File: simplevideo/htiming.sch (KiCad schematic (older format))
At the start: 4 parts, among them U14 CD74HC40103, U15 CD74HC40103, U16 CD74HC40103, U17 74LS74

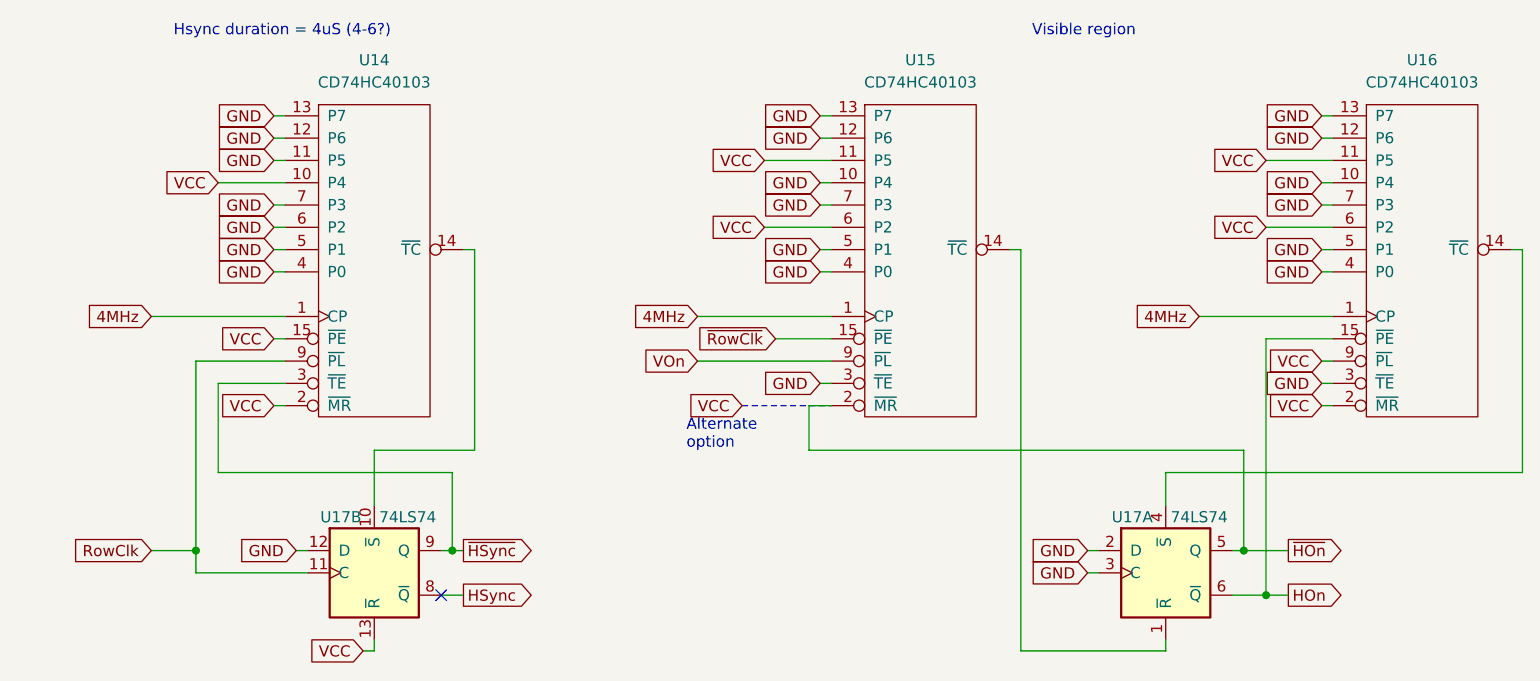
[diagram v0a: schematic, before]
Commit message: Fixed various issues discovered during building and testing
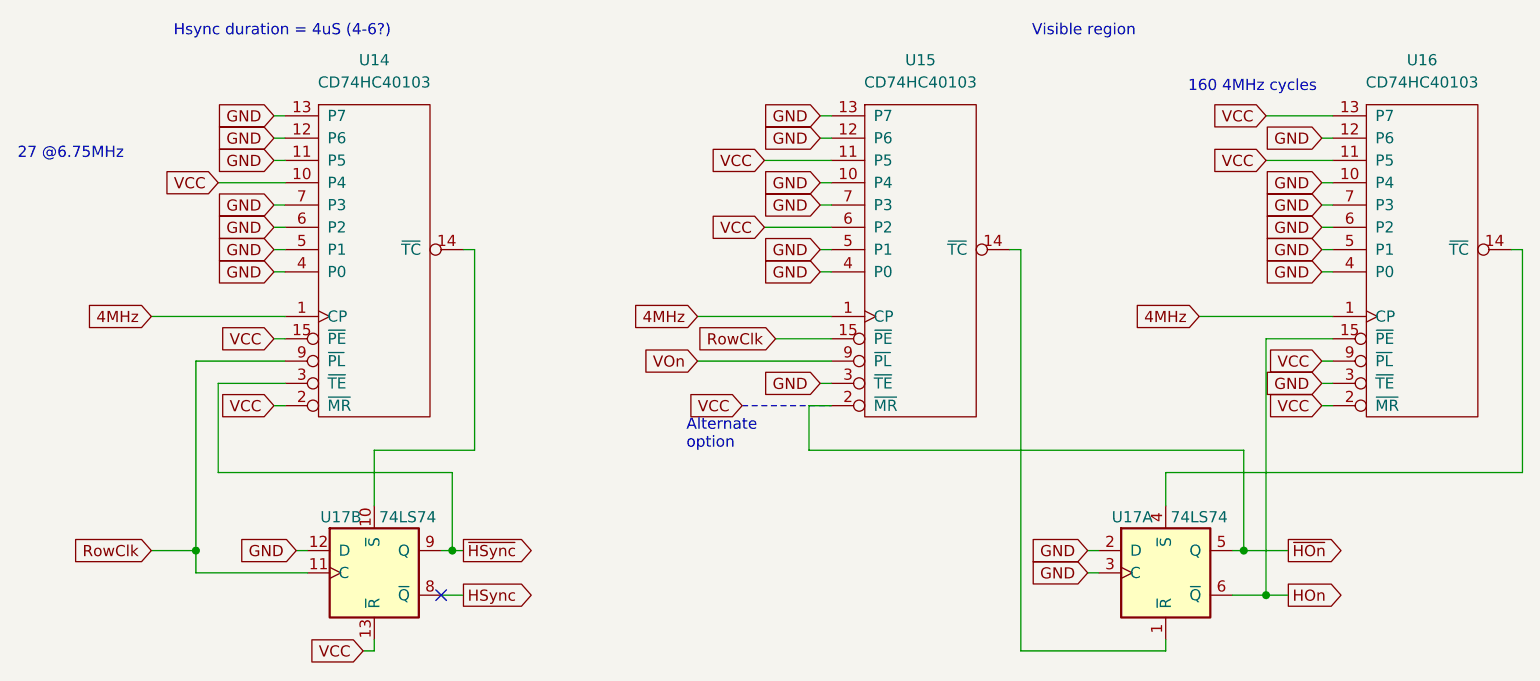
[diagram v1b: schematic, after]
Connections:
- net ~RowClk is gone; now on net RowClk: U15.15 (~PE)
- net GND: now also U16.6 (P2); no longer U16.13 (P7)
- net VCC: now also U16.13 (P7); no longer U16.6 (P2)
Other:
- note added: "160 4MHz cycles"
- note added: "27 @6.75MHz"
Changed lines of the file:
@@
 Text GLabel 6250 1450 0    50   Input ~ 0
 VCC
-Text GLabel 6250 1750 0    50   Input ~ 0
-VCC
-Text GLabel 6500 1650 0    50   Input ~ 0
-GND
-Text GLabel 6500 1550 0    50   Input ~ 0
-GND
-Text GLabel 6500 1950 0    50   Input ~ 0
-GND
-Text GLabel 6500 1350 0    50   Input ~ 0
-GND
-Text GLabel 6500 1250 0    50   Input ~ 0
-GND
-Text GLabel 6500 1850 0    50   Input ~ 0
-GND
 Wire Wire Line
 	7400 1850 7400 2850
@@
 	6500 1850 6550 1850
 Wire Wire Line
-	6250 1750 6550 1750
+	6500 1750 6550 1750
 Wire Wire Line
 	6500 1650 6550 1650
@@
 	6500 1350 6550 1350
 Wire Wire Line
-	6500 1250 6550 1250
+	6250 1250 6550 1250
 Wire Wire Line
 	6550 1950 6500 1950
@@
 VOn
 Text GLabel 4050 2250 0    50   Input ~ 0
-~RowClk
+RowClk
 Wire Notes Line
 	3900 2550 4300 2550
@@
 	6350 3200 6150 3200
 Connection ~ 6150 3200
+Text Notes 650  1450 0    50   ~ 0
+27 @6.75MHz
+Text GLabel 6250 1250 0    50   Input ~ 0
+VCC
+Text GLabel 6500 1350 0    50   Input ~ 0
+GND
+Text GLabel 6500 1550 0    50   Input ~ 0
+GND
+Text GLabel 6500 1650 0    50   Input ~ 0
+GND
+Text GLabel 6500 1850 0    50   Input ~ 0
+GND
+Text GLabel 6500 1950 0    50   Input ~ 0
+GND
+Text GLabel 6500 1750 0    50   Input ~ 0
+GND
+Text Notes 5900 1150 0    50   ~ 0
+160 4MHz cycles
 $EndSCHEMATC
